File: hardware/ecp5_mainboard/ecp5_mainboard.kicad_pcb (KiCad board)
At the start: 8 copper layers, 158.1 x 111.2 mm, 508 parts, among them J1 12V_EXT, J10 UART, J11 FLASH, J12 JTAG, J13 Micro_SD_Card, J2 USB_B_Micro, J3 HDMI_A, J4 USB_A, J5 EXT0, J6 EXT1, J7 EXT2, J8 EXT3, J9 PMOD_01, P1 SATA, P2 SATA, P3 PCIe_x4_EDGE, P4 JK0654219NL, Q1 BSH111BKR, Q2 BC850, Q3 BSH111BKR, Q4 BC850, Q5 BSH111BKR, Q6 BSH111BKR, Q7 BSH111BKR, Q8 BSH111BKR, Q9 BSH111BKR, SW1 CHP-081TA, SW2 SW_Push, SW3 SW_Push, SW4 SW_Push, SW5 SW_Push, SW6 SW_Push, U1 MAX811MEUS-T, U10 TPS62823, U12 93AA46B_OT, U13 FT2232H, U14 XUL535150.000JS6I8, U15 ECP5UM5G_85_CABGA756, U16 5P49V6965, U17 TPS2041B, U18 PCA9306, U19 TFP410, U2 LM3880, U20 TPS2041B, U21 KSZ9031RNXCA, U22 USB3300-EZK, U23 AS4C256M16D3, U24 AS4C256M16D3, U25 TPS51200DRC, U26 XL_XO_LVDS, U27 W25Q, U3 TLV75712PDR, U4 TPS565208, U5 LM21212-2, U6 TLV75712PDR, U7 TPS62823, U8 TPS62823, U9 TPS62823, X1 XO32, Y1 25MHz, Y2 25MHz, Y3 24MHz

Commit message: hardware/mainboard: Swapping DDR3 groups
Signed-off-by: David Shah <dave@ds0.me>
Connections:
- U15 pad AB26: DDR3_RAS -> DDR3_DQ27
- U15 pad AB27: DDR3_ODT -> DDR3_DQS3-
- U15 pad AB28: DDR3_CKE -> DDR3_DQS3+
- U15 pad AC26: DDR3_WE -> DDR3_DQ24
- U15 pad AC27: DDR3_CS -> DDR3_DQ25
- U15 pad AD26: DDR3_RESET -> Net-(U15-PadAD26)
- U15 pad AD27: DDR3_CLK+ -> Net-(U15-PadAD27)
- U15 pad AE27: DDR3_CLK- -> Net-(U15-PadAE27)
- U15 pad B32: DDR3_DQS2+ -> DDR3_A8
- U15 pad C31: DDR3_DQS2- -> DDR3_A6
- U15 pad C32: DDR3_DQ18 -> DDR3_A3
- U15 pad D29: Net-(U15-PadD29) -> DDR3_A12
- U15 pad D30: DDR3_DQ21 -> DDR3_A7
- U15 pad D31: DDR3_DQ20 -> DDR3_A5
- U15 pad D32: DDR3_DQ16 -> DDR3_A1
- U15 pad E29: DDR3_DQ23 -> DDR3_A10
- U15 pad E30: DDR3_DQ17 -> DDR3_A2
- U15 pad E32: Net-(U15-PadE32) -> DDR3_A13
- U15 pad F28: DDR3_DQ22 -> DDR3_A9
- U15 pad F29: DDR3_DM2 -> DDR3_A11
- U15 pad F30: DDR3_DQ19 -> DDR3_A4
- U15 pad F31: Net-(U15-PadF31) -> DDR3_A0
- U15 pad F32: Net-(U15-PadF32) -> DDR3_A14
- U15 pad H30: DDR3_DQ15 -> DDR3_RAS
- U15 pad H31: Net-(U15-PadH31) -> DDR3_BA1
- U15 pad H32: Net-(U15-PadH32) -> DDR3_BA0
- U15 pad J29: DDR3_DQ10 -> DDR3_RESET
- U15 pad J30: DDR3_DM1 -> DDR3_BA2
- U15 pad J32: DDR3_DQS1- -> DDR3_WE
- U15 pad K26: Net-(U15-PadK26) -> DDR3_DQ15
- U15 pad K28: Net-(U15-PadK28) -> DDR3_DM1
- U15 pad K29: DDR3_DQ8 -> Net-(U15-PadK29)
- U15 pad K30: DDR3_DQ14 -> DDR3_CAS
- U15 pad K31: DDR3_DQS1+ -> DDR3_CS
- U15 pad K32: DDR3_DQ13 -> DDR3_CKE
- U15 pad L26: Net-(U15-PadL26) -> DDR3_DQ13
- U15 pad L27: Net-(U15-PadL27) -> DDR3_DQ12
- U15 pad L29: Net-(U15-PadL29) -> DDR3_DQ14
- U15 pad L30: DDR3_DQ9 -> DDR3_CLK-
- U15 pad L31: DDR3_DQ11 -> DDR3_CLK+
- U15 pad L32: DDR3_DQ12 -> DDR3_ODT
- U15 pad N26: Net-(U15-PadN26) -> DDR3_DQ9
- U15 pad N27: Net-(U15-PadN27) -> DDR3_DQ11
- U15 pad N29: DDR3_DQS0- -> DDR3_DQS1-
- U15 pad N30: DDR3_DQS0+ -> DDR3_DQS1+
- U15 pad N32: DDR3_A11 -> Net-(U15-PadN32)
- U15 pad P26: Net-(U15-PadP26) -> DDR3_DQ8
- U15 pad P27: Net-(U15-PadP27) -> DDR3_DQ10
- U15 pad P32: DDR3_A9 -> DDR3_DQ23
- U15 pad R27: DDR3_DM3 -> DDR3_DQ1
- U15 pad R29: DDR3_DQS3+ -> DDR3_DQS0+
- U15 pad R32: DDR3_A7 -> DDR3_DQS2+
- U15 pad T27: DDR3_DQ30 -> DDR3_DQ7
- U15 pad T28: DDR3_DQS3- -> DDR3_DQS0-
- U15 pad T29: DDR3_DQ28 -> DDR3_DQ5
- U15 pad T30: DDR3_A12 -> Net-(U15-PadT30)
- U15 pad T31: DDR3_A5 -> DDR3_DQS2-
- U15 pad T32: DDR3_A3 -> DDR3_DQ19
- U15 pad U26: DDR3_DQ29 -> DDR3_DQ6
- U15 pad U27: DDR3_DQ31 -> DDR3_DM0
- U15 pad U28: DDR3_DQ27 -> DDR3_DQ4
- U15 pad U29: DDR3_DQ26 -> DDR3_DQ3
- U15 pad U30: DDR3_A8 -> DDR3_DQ22
- U15 pad U31: DDR3_A10 -> DDR3_DM2
- U15 pad U32: DDR3_A1 -> DDR3_DQ17
- U15 pad V26: DDR3_DQ24 -> DDR3_DQ0
- U15 pad V27: DDR3_DQ25 -> DDR3_DQ2
- U15 pad V32: DDR3_A2 -> DDR3_DQ18
- U15 pad W28: DDR3_BA1 -> DDR3_DQ29
- U15 pad W29: DDR3_CAS -> DDR3_DQ26
- U15 pad W30: DDR3_A6 -> DDR3_DQ21
- U15 pad W32: DDR3_A0 -> DDR3_DQ16
- U15 pad Y26: DDR3_A14 -> DDR3_DM3
- U15 pad Y27: DDR3_BA0 -> DDR3_DQ30
- U15 pad Y28: DDR3_A13 -> DDR3_DQ31
- U15 pad Y29: DDR3_BA2 -> DDR3_DQ28
- U15 pad Y30: DDR3_A4 -> DDR3_DQ20

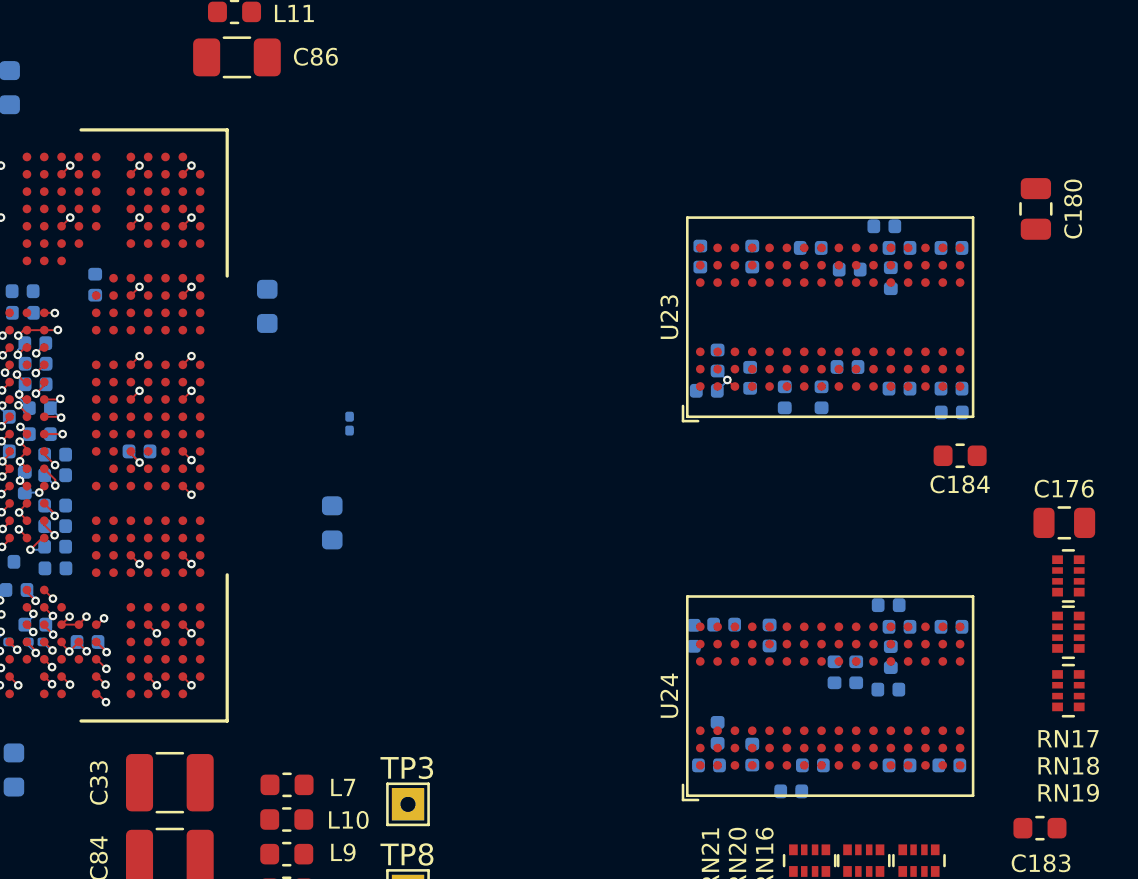
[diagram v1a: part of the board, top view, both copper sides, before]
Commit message: hardware/mainboard: DDR3 Address routing
Signed-off-by: David Shah <dave@ds0.me>
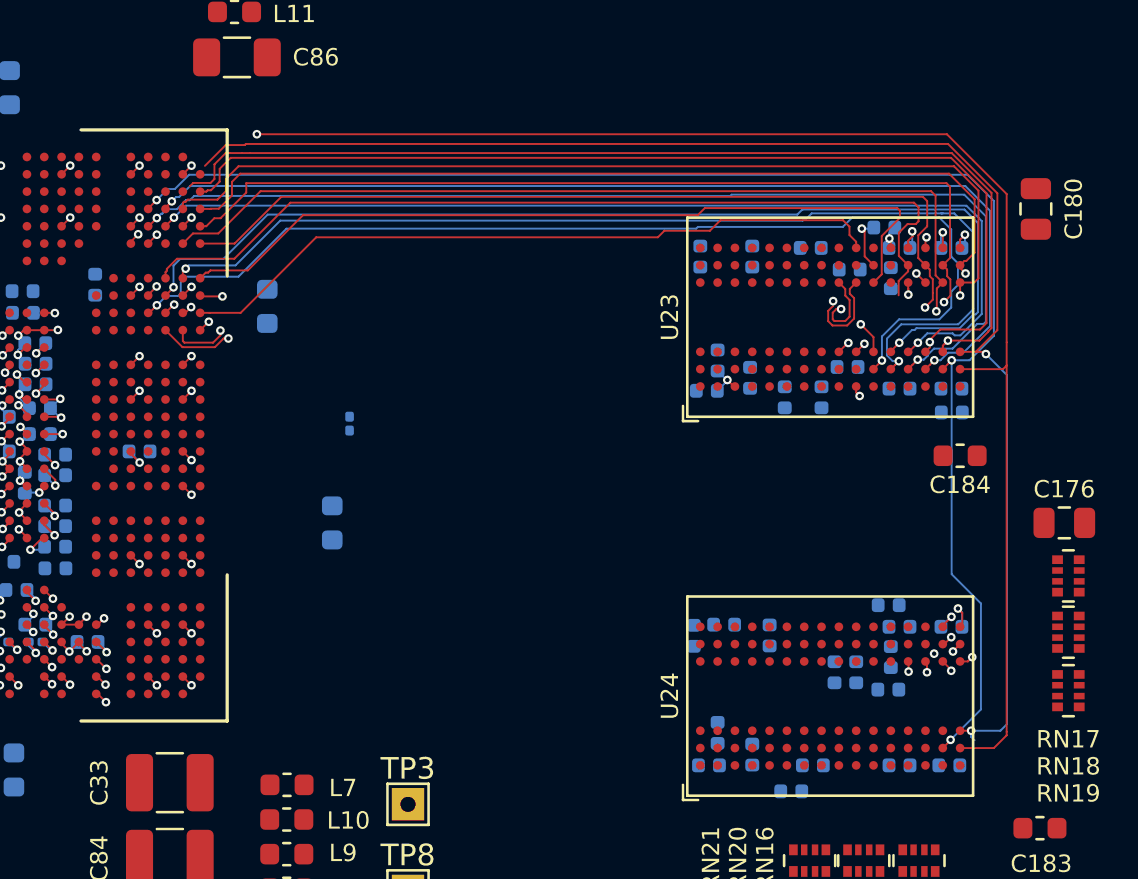
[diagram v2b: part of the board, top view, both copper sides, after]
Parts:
- moved R80 0.06 mm to (168.0, 60.9)
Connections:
- U15 pad B32: DDR3_A8 -> DDR3_A13
- U15 pad C31: DDR3_A6 -> DDR3_A9
- U15 pad C32: DDR3_A3 -> DDR3_A2
- U15 pad D29: DDR3_A12 -> DDR3_A7
- U15 pad D30: DDR3_A7 -> DDR3_A5
- U15 pad D31: DDR3_A5 -> DDR3_A14
- U15 pad D32: DDR3_A1 -> DDR3_A8
- U15 pad E29: DDR3_A10 -> DDR3_A3
- U15 pad E30: DDR3_A2 -> DDR3_A0
- U15 pad E32: DDR3_A13 -> DDR3_A6
- U15 pad F28: DDR3_A9 -> DDR3_A1
- U15 pad F29: DDR3_A11 -> DDR3_A12
- U15 pad F30: DDR3_A4 -> Net-(U15-PadF30)
- U15 pad F31: DDR3_A0 -> DDR3_A11
- U15 pad F32: DDR3_A14 -> DDR3_A4
- U15 pad H30: DDR3_RAS -> DDR3_BA1
- U15 pad H31: DDR3_BA1 -> DDR3_BA0
- U15 pad H32: DDR3_BA0 -> DDR3_A10
- U15 pad J29: DDR3_RESET -> DDR3_ODT
- U15 pad K29: Net-(U15-PadK29) -> DDR3_CS
- U15 pad K30: DDR3_CAS -> DDR3_RAS
- U15 pad K31: DDR3_CS -> DDR3_CAS
- U15 pad L32: DDR3_ODT -> DDR3_RESET
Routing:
- net DDR3_RESET: track 0.00 -> 76.0 mm, vias 0 -> 2
- net DDR3_A7: track 0.00 -> 68.7 mm, vias 0 -> 3
- net DDR3_A1: track 0.00 -> 67.7 mm, vias 0 -> 3
- net DDR3_A13: track 0.00 -> 67.2 mm, vias 0 -> 2
- net DDR3_A12: track 0.00 -> 65.6 mm, vias 0 -> 3
- net DDR3_A14: track 0.00 -> 61.7 mm, vias 0 -> 2
- net DDR3_A8: track 0.00 -> 59.9 mm, vias 0 -> 2
- net DDR3_A11: track 0.00 -> 59.8 mm, vias 0 -> 2
- net DDR3_A6: track 0.00 -> 58.9 mm, vias 0 -> 2
- net DDR3_A4: track 0.00 -> 58.3 mm, vias 0 -> 2
- net DDR3_A3: track 0.00 -> 49.1 mm, vias 0 -> 2
- net DDR3_BA2: track 0.00 -> 48.9 mm, vias 0 -> 2
- net DDR3_CS: track 0.00 -> 48.7 mm, vias 0 -> 2
- net DDR3_BA0: track 0.00 -> 48.4 mm, vias 0 -> 2
- net DDR3_ODT: track 0.00 -> 48.2 mm, vias 0 -> 2
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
